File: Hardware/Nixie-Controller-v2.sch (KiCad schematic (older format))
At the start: 220 parts, among them J7 12V DC JACK, U1 MAX1771, U10 74HC4067, U11 M41T01, U12 STM32F103C8, U13 OPA180, U14 74HC4067, U15 OPA180, U16 74HC4067, U17 OPA180, U18 74HC4067, U19 OPA180, U2 BH2226, U20 74HC4067, U21 OPA180, U22 74HC4067, U3 74HC595, U4 74HC595, U5 74HC595, U6 SN74LVCC3245A, U7 NCP1117-5.0, U8 NCP1117-3.3, U9 OPA180, Y1 32.768KHz

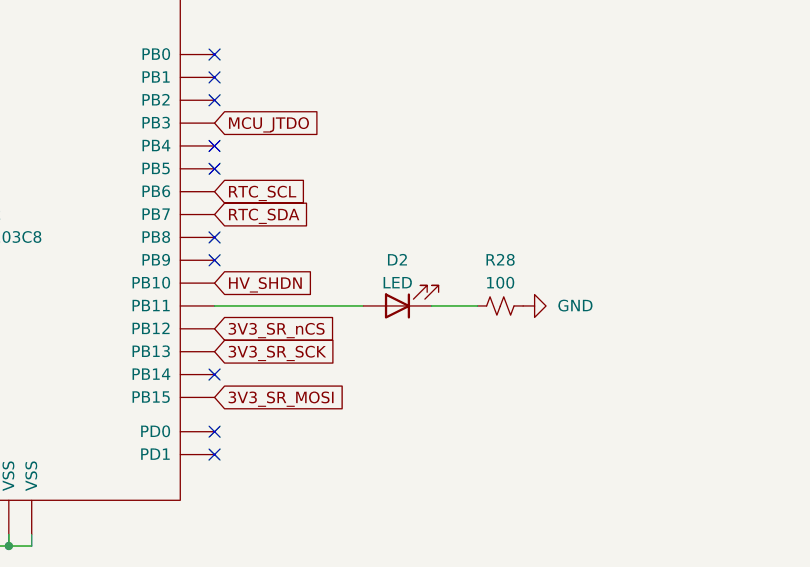
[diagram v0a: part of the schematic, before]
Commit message: Remove status LED
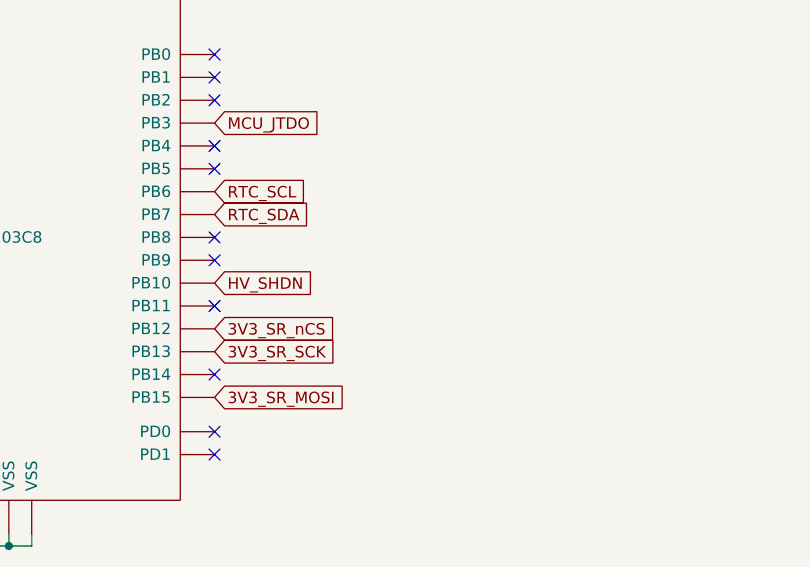
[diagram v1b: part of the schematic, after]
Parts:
- removed D2: LED, Diode_SMD:D_0603_1608Metric, symbol Device:LED
- removed R28: 100, Resistor_SMD:R_0402_1005Metric, symbol Device:R_Small_US
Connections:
- no-connect marks 77 -> 78
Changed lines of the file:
@@
-$EndComp
-Wire Wire Line
-	18700 9200 18050 9200
-Wire Wire Line
-	19200 9200 19000 9200
-$Comp
-L power:GND #PWR0124
-U 1 1 61A95A14
-P 19400 9200
-F 0 "#PWR0124" H 19400 8950 50  0001 C CNN
-F 1 "GND" V 19400 9050 50  0000 R CNN
-F 2 "" H 19400 9200 50  0001 C CNN
-F 3 "" H 19400 9200 50  0001 C CNN
-	1    19400 9200
-	0    -1   -1   0
-$EndComp
-$Comp
-L Device:R_Small_US R28
-U 1 1 6186EA54
-P 19300 9200
-F 0 "R28" V 19100 9200 50  0000 C CNN
-F 1 "100" V 19200 9200 50  0000 C CNN
-F 2 "Resistor_SMD:R_0402_1005Metric" H 19300 9200 50  0001 C CNN
-F 3 "~" H 19300 9200 50  0001 C CNN
-F 4 "Yageo" H 19300 9200 50  0001 C CNN "Manufacturer"
-F 5 "RC0402FR-07100RL" H 19300 9200 50  0001 C CNN "Part#"
-	1    19300 9200
-	0    1    1    0
-$EndComp
-$Comp
-L Device:LED D2
-U 1 1 6186BE38
-P 18850 9200
-F 0 "D2" H 18850 9000 50  0000 C CNN
-F 1 "LED" H 18850 9100 50  0000 C CNN
-F 2 "Diode_SMD:D_0603_1608Metric" H 18850 9200 50  0001 C CNN
-F 3 "~" H 18850 9200 50  0001 C CNN
-F 4 "Rohm Semi" H 18850 9200 50  0001 C CNN "Manufacturer"
-F 5 "SML-D12U1WT86" H 18850 9200 50  0001 C CNN "Part#"
-	1    18850 9200
-	-1   0    0    1
 $EndComp
 Wire Wire Line
@@
 Text Notes 32600 11400 2    197  ~ 39
 WIFI
+NoConn ~ 18050 9200
 $EndSCHEMATC
